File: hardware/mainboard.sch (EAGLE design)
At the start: 34 parts, among them IC1 ESP-12E/F, Q1 BC847BS, Q2 BC847BS, Q3 BC847BS

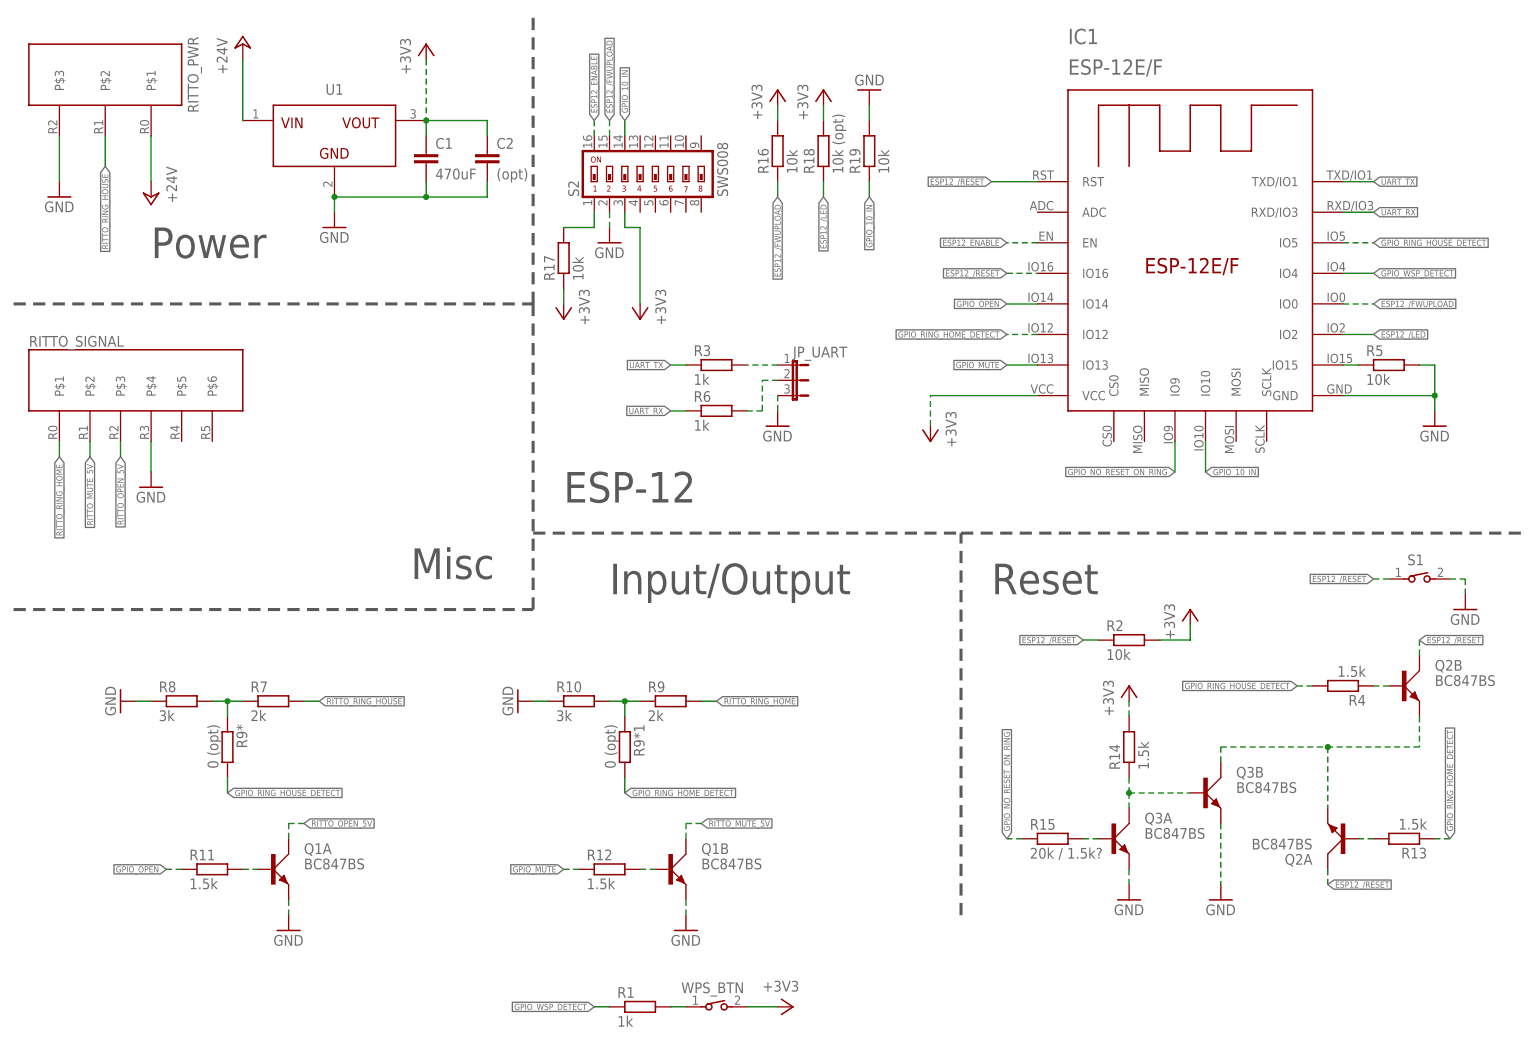
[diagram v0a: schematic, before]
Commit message: Checkpoint commit for board file
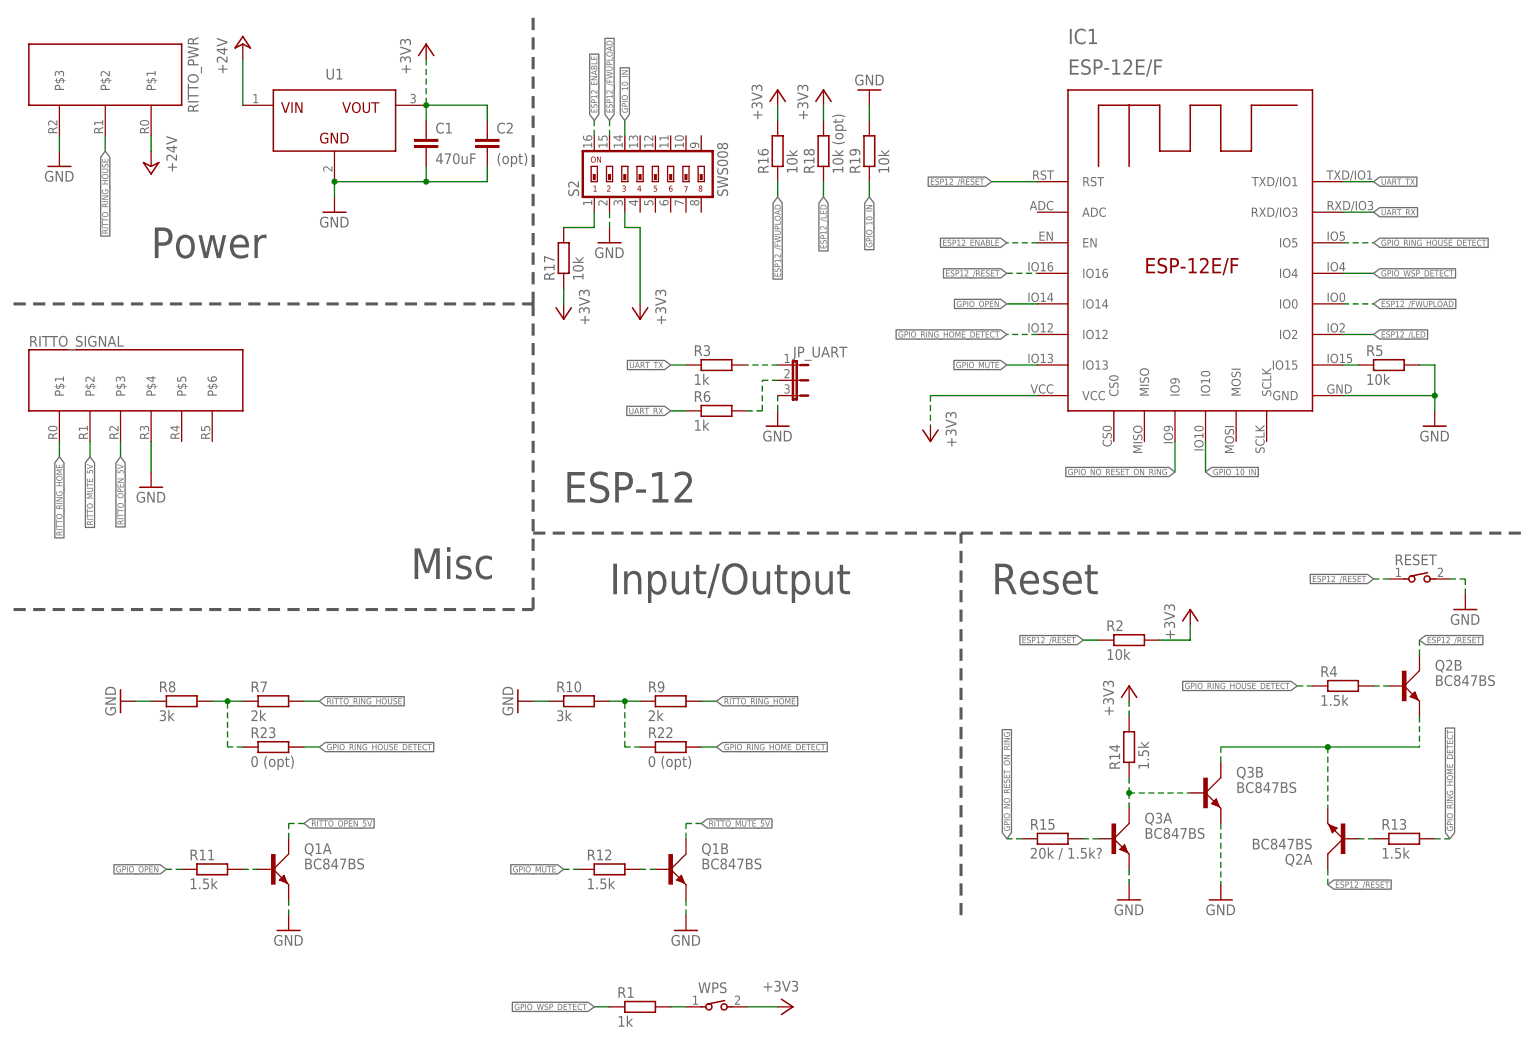
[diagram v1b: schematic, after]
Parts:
- removed R9*, R9*1: 0 (opt), rcl:R-EU_R1206
- added R22, R23: 0 (opt), rcl:R-EU_R1206
- renumbered S1 to RESET, WPS_BTN to WPS
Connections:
- removed net N$12: Q2A.B, R13.2
- removed net N$13: Q2B.B, R4.1
- new net N$8: Q2B.B, R4.2
- new net N$9: Q2A.B, R13.1
- net GPIO_RING_HOME_DETECT: now also R13.2, R22.2; no longer R13.1, R9*1.2
- net GPIO_RING_HOUSE_DETECT: now also R23.2, R4.1; no longer R4.2, R9*.2
- net N$5: now also R23.1; no longer R9*.1
- net N$6: now also R22.1; no longer R9*1.1
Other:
- moved on the sheet: C1, C2, R13, R4, U1
